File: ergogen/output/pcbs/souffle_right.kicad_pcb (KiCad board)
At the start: 2 copper layers, 135.6 x 116.1 mm, 60 parts

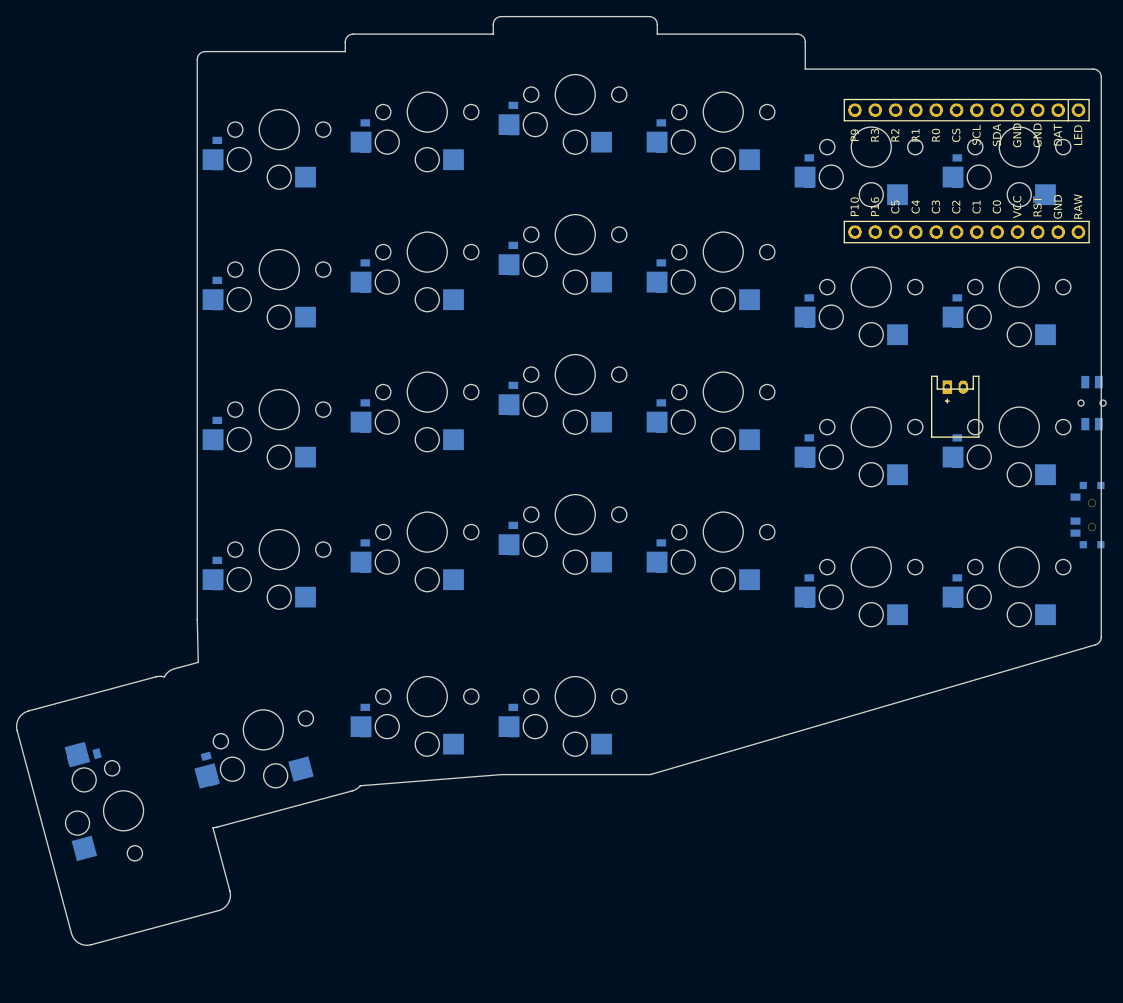
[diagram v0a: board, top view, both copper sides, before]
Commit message: feat: left hand redesign
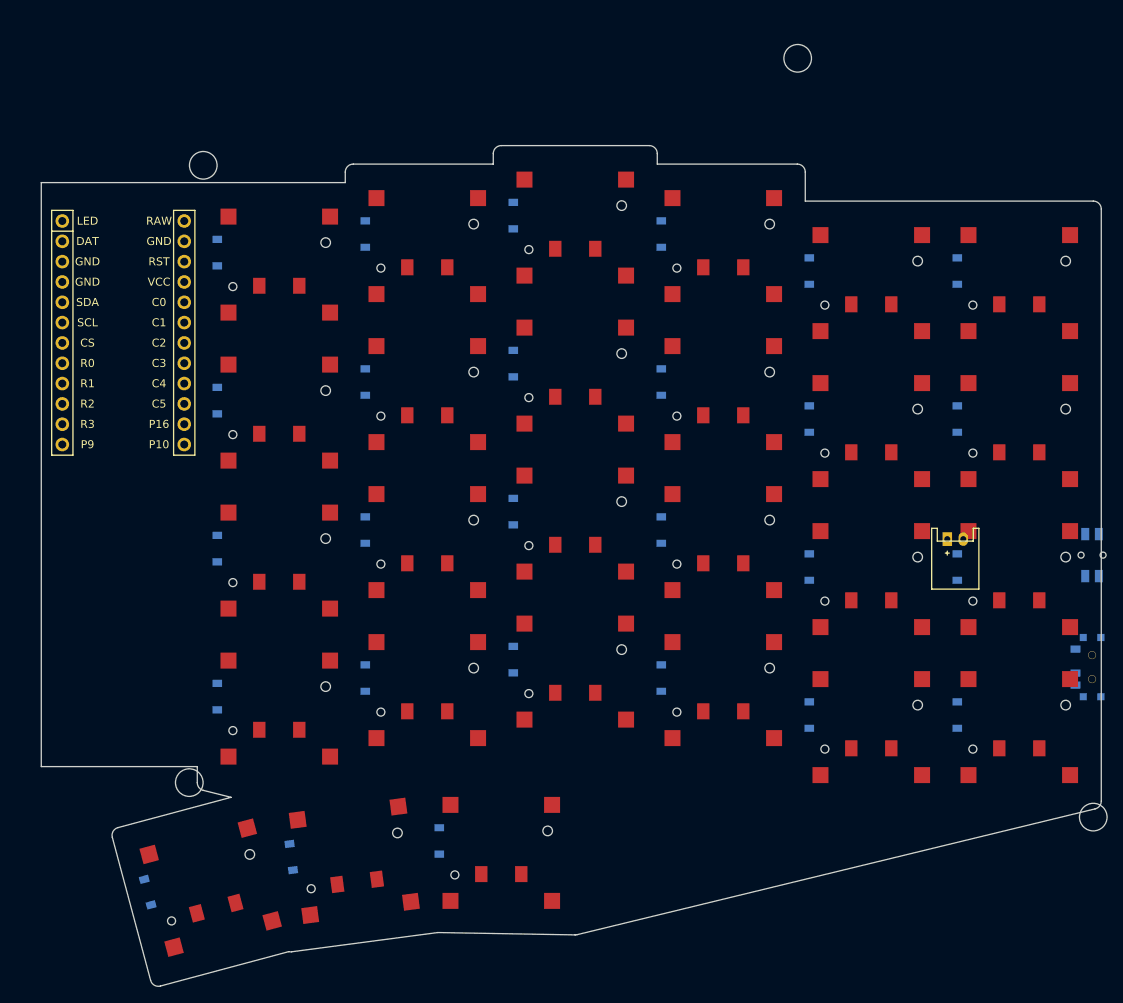
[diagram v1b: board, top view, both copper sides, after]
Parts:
- removed D28: , ceoloide:diode_tht_sod123
- removed S28: , ceoloide:switch_choc_v1_v2
- added MH1: , ceoloide:mounting_hole_npth, F.Cu at (337.3, 36.4)
- added MH2: , ceoloide:mounting_hole_npth, F.Cu at (263.0, 49.8)
- added MH3: , ceoloide:mounting_hole_npth, F.Cu at (374.2, 131.2)
- added MH4: , ceoloide:mounting_hole_npth, F.Cu at (261.2, 126.9)
- S1, S10, S11, S12, S13, S14, S15, S16, S17, S18, S19, S2, S20, S21, S22, S23, S24, S25, S26, S27, S3, S4, S5, S6, S7, S8, S9: footprint ceoloide:switch_choc_v1_v2 -> CPG1316S01D02_mikeholscher; moved to F.Cu
- moved MCU1 108.4 mm to (253.0, 69.4), turned to 0 degrees
- moved S26 22.5 mm to (281.9, 136.7), turned to 7.5 degrees
- moved S25 21.6 mm to (300.2, 135.7), turned to 0 degrees
- moved S27 20.8 mm to (263.9, 140.1), turned to 15 degrees
- moved S1 20.0 mm to (365.0, 120.0), turned to 0 degrees
- moved S5 20.0 mm to (346.5, 120.0), turned to 0 degrees
- moved S21 19.9 mm to (272.5, 117.7), turned to 0 degrees
- moved S17 19.8 mm to (291.0, 115.4), turned to 0 degrees
- moved S9 19.8 mm to (328.0, 115.4), turned to 0 degrees
- moved S13 19.6 mm to (309.5, 113.1), turned to 0 degrees
- moved D26 19.4 mm to (274.0, 136.2), turned to -82.5 degrees
- moved B1 19.0 mm to (374.1, 98.5)
- moved JST1 19.0 mm to (357.0, 96.5)
- moved S2 19.0 mm to (365.0, 101.5), turned to 0 degrees
- moved S6 19.0 mm to (346.5, 101.5), turned to 0 degrees
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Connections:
- D26 pad 2: mirror_outward_home -> mirror_middle_home
- D27 pad 2: mirror_small_thumbkey_home -> mirror_outward_home
- S1 pad 1: C0 -> mirror_outer_bottom
- S1 pad 2: mirror_outer_bottom -> C0
- S10 pad 1: C2 -> mirror_ring_home
- S10 pad 2: mirror_ring_home -> C2
- S11 pad 1: C2 -> mirror_ring_top
- S11 pad 2: mirror_ring_top -> C2
- S12 pad 1: C2 -> mirror_ring_number
- S12 pad 2: mirror_ring_number -> C2
- S13 pad 1: C3 -> mirror_middle_bottom
- S13 pad 2: mirror_middle_bottom -> C3
- S14 pad 1: C3 -> mirror_middle_home
- S14 pad 2: mirror_middle_home -> C3
- S15 pad 1: C3 -> mirror_middle_top
- S15 pad 2: mirror_middle_top -> C3
- S16 pad 1: C3 -> mirror_middle_number
- S16 pad 2: mirror_middle_number -> C3
- S17 pad 1: C4 -> mirror_index_bottom
- S17 pad 2: mirror_index_bottom -> C4
- S18 pad 1: C4 -> mirror_index_home
- S18 pad 2: mirror_index_home -> C4
- S19 pad 1: C4 -> mirror_index_top
- S19 pad 2: mirror_index_top -> C4
- S2 pad 1: C0 -> mirror_outer_home
- S2 pad 2: mirror_outer_home -> C0
- S20 pad 1: C4 -> mirror_index_number
- S20 pad 2: mirror_index_number -> C4
- S21 pad 1: C5 -> mirror_inner_bottom
- S21 pad 2: mirror_inner_bottom -> C5
- S22 pad 1: C5 -> mirror_inner_home
- S22 pad 2: mirror_inner_home -> C5
- S23 pad 1: C5 -> mirror_inner_top
- S23 pad 2: mirror_inner_top -> C5
- S24 pad 1: C5 -> mirror_inner_number
- S24 pad 2: mirror_inner_number -> C5
- S25 pad 1: C2 -> mirror_inward_home
- S25 pad 2: mirror_inward_home -> C2
- S26 pad 1: C3 -> mirror_middle_home
- S26 pad 2: mirror_outward_home -> C4
- S27 pad 1: C4 -> mirror_outward_home
- S27 pad 2: mirror_small_thumbkey_home -> C5
- S3 pad 1: C0 -> mirror_outer_top
- S3 pad 2: mirror_outer_top -> C0
- S4 pad 1: C0 -> mirror_outer_number
- S4 pad 2: mirror_outer_number -> C0
- S5 pad 1: C1 -> mirror_pinky_bottom
- S5 pad 2: mirror_pinky_bottom -> C1
- S6 pad 1: C1 -> mirror_pinky_home
- S6 pad 2: mirror_pinky_home -> C1
- S7 pad 1: C1 -> mirror_pinky_top
- S7 pad 2: mirror_pinky_top -> C1
- S8 pad 1: C1 -> mirror_pinky_number
- S8 pad 2: mirror_pinky_number -> C1
- S9 pad 1: C2 -> mirror_ring_bottom
- S9 pad 2: mirror_ring_bottom -> C2
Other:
- board size 135.6 x 116.1 mm -> 132.5 x 105.1 mm
